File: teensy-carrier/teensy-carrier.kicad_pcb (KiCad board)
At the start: 2 copper layers, 56 x 18 mm, 3 parts, among them J1 Conn_01x02_Male, J2 Conn_01x15_Female, U1 Teensy3.2

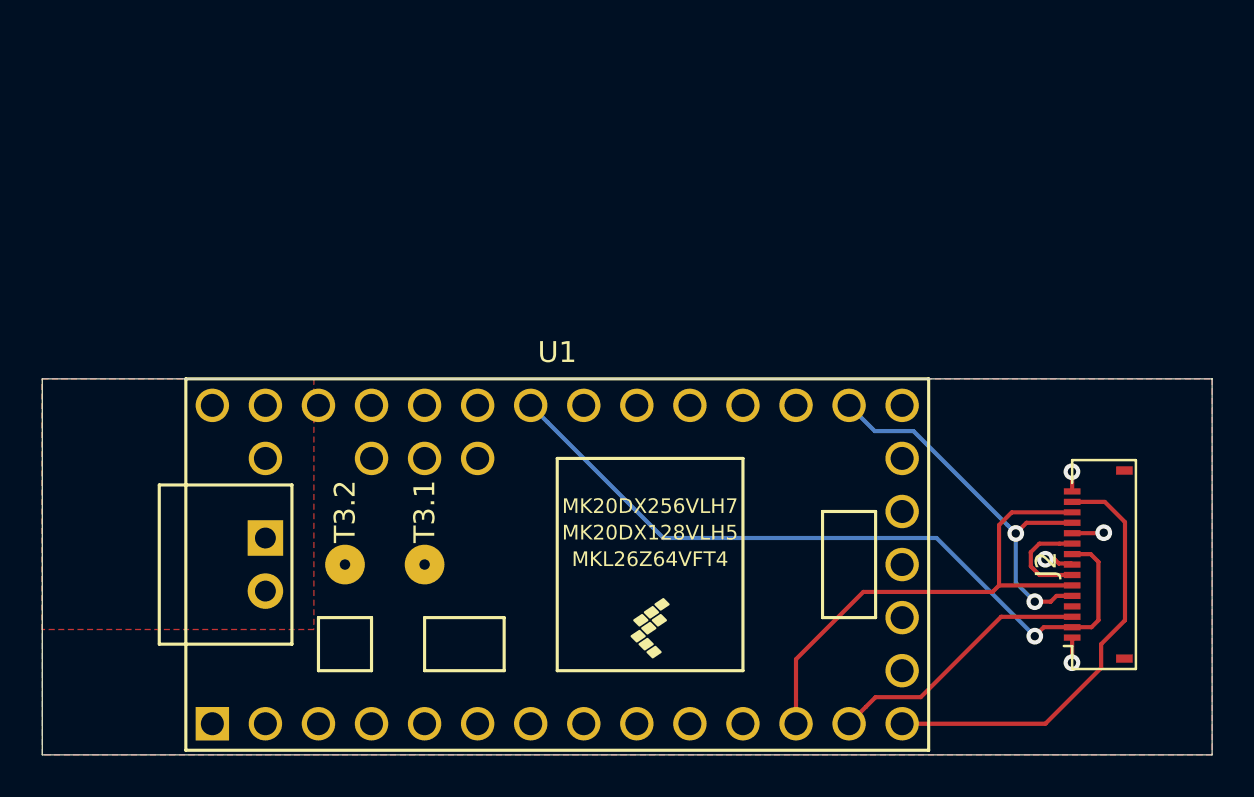
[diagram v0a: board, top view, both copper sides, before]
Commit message: work on teensy-carrier
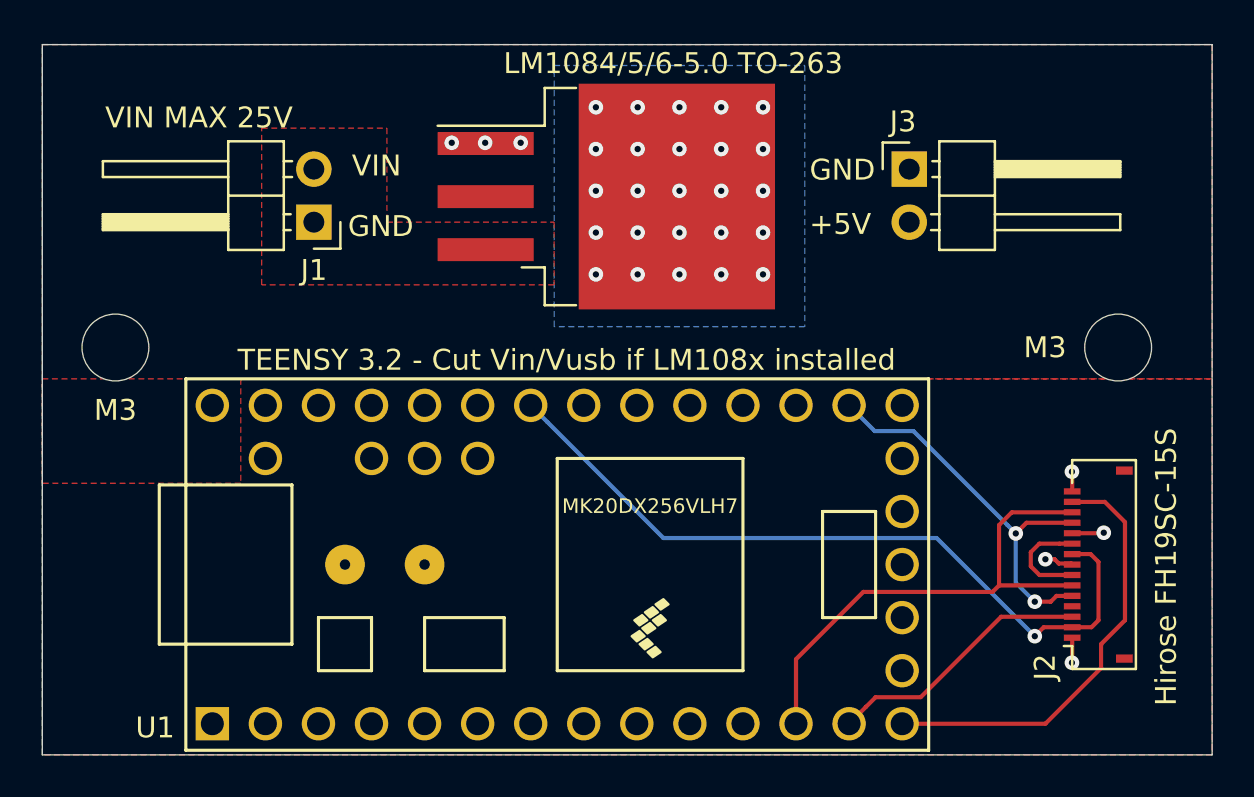
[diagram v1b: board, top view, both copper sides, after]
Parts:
- added J3: Conn_01x02_Female, Connector_PinHeader_2.54mm:PinHeader_1x02_P2.54mm_Horizontal, F.Cu at (709.0, 371.0)
- added REF**: MountingHole_3.2mm_M3, MountingHole:MountingHole_3.2mm_M3, F.Cu at (671.0, 379.5)
- added REF**: MountingHole_3.2mm_M3, MountingHole:MountingHole_3.2mm_M3, F.Cu at (719.0, 379.5)
- added REF**: bear, teensy:bear, B.Cu at (672.7, 366.5)
- added U2: LM1084-5.0, Package_TO_SOT_SMD:TO-263-3_TabPin2, F.Cu at (694.5, 372.3)
- J1: moved to F.Cu
- moved J1 15.3 mm to (680.5, 373.5)
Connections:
- J1 pad 2: +5V -> Net-(J1-Pad2)
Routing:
- net GND: vias 4 -> 7
- net +5V: vias 0 -> 25
- added copper zone on B.Cu, net +5V
- added copper zone on F.Cu, net Net-(J1-Pad2)
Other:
- board size 56 x 18 mm -> 56 x 34 mm
- board text added: "+5V"
- board text added: "GND"
- board text added: "Hirose FH19SC-15S"
- board text added: "LM1084/5/6-5.0 TO-263"
- board text added: "M3"
- board text added: "TEENSY 3.2 - Cut Vin/Vusb if LM108x installed"
- board text added: "UVTV Control & Power v1 SB Powell PhD samuel.powell@uq.edu.au"
- board text added: "VIN"
- board text added: "VIN MAX 25V"
